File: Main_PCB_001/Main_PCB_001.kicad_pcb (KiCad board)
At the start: 4 copper layers, 55 x 15 mm, 65 parts, among them IC1 FDN8601, IC2 FDN8601, IC3 TPS40211QDGQRQ1, IC4 PAM2863ECR, IC5 FDN8601, IC6 ZXTR2105FQ-7, U1 ATtiny25-20S, U2 Mounting_Hole_M2, U3 Mounting_Hole_M2, U4 Mounting_Hole_M2, U5 Mounting_Hole_M2

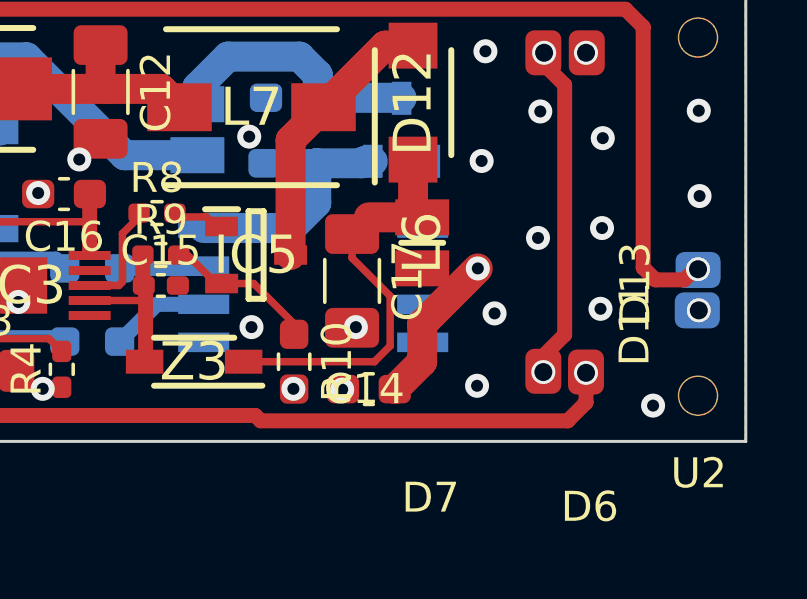
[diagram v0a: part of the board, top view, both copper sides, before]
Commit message: Corrections 001
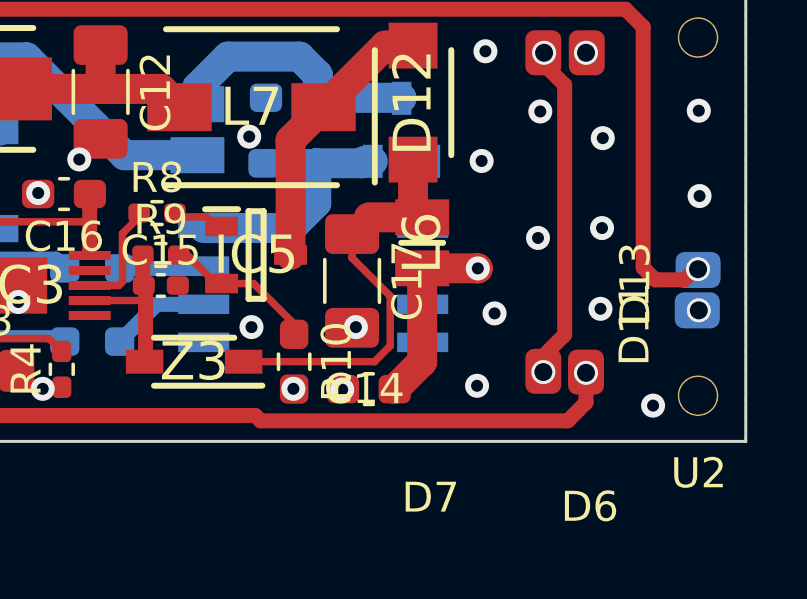
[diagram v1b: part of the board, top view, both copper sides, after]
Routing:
- net Net-(C14-Pad1): track 15.5 -> 16.6 mm
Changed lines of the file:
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@@
   (segment (start 133.7564 102.2958) (end 135.522 102.2958) (width 1) (layer "F.Cu") (net 10))
   (segment (start 135.522 102.2958) (end 136.1316 102.9054) (width 1) (layer "F.Cu") (net 10))
-  (segment (start 146.0754 108.2802) (end 144.2212 110.1344) (width 1) (layer "F.Cu") (net 11))
-  (segment (start 144.2212 110.1344) (end 144.2212 111.3879) (width 1) (layer "F.Cu") (net 11))
+  (segment (start 144.2212 108.2766) (end 144.2212 111.3879) (width 1) (layer "F.Cu") (net 11))
   (segment (start 144.2212 111.3879) (end 143.3057 112.3034) (width 1) (layer "F.Cu") (net 11))
+  (segment (start 146.0754 108.2802) (end 146.0718 108.2766) (width 1) (layer "F.Cu") (net 11))
+  (segment (start 146.0718 108.2766) (end 144.2212 108.2766) (width 1) (layer "F.Cu") (net 11))
   (via (at 146.0754 108.2802) (size 0.8) (drill 0.4) (layers "F.Cu" "B.Cu") (net 11))
   (via (at 149.6822 101.092) (size 0.8) (drill 0.6) (layers "F.Cu" "B.Cu") (net 11))

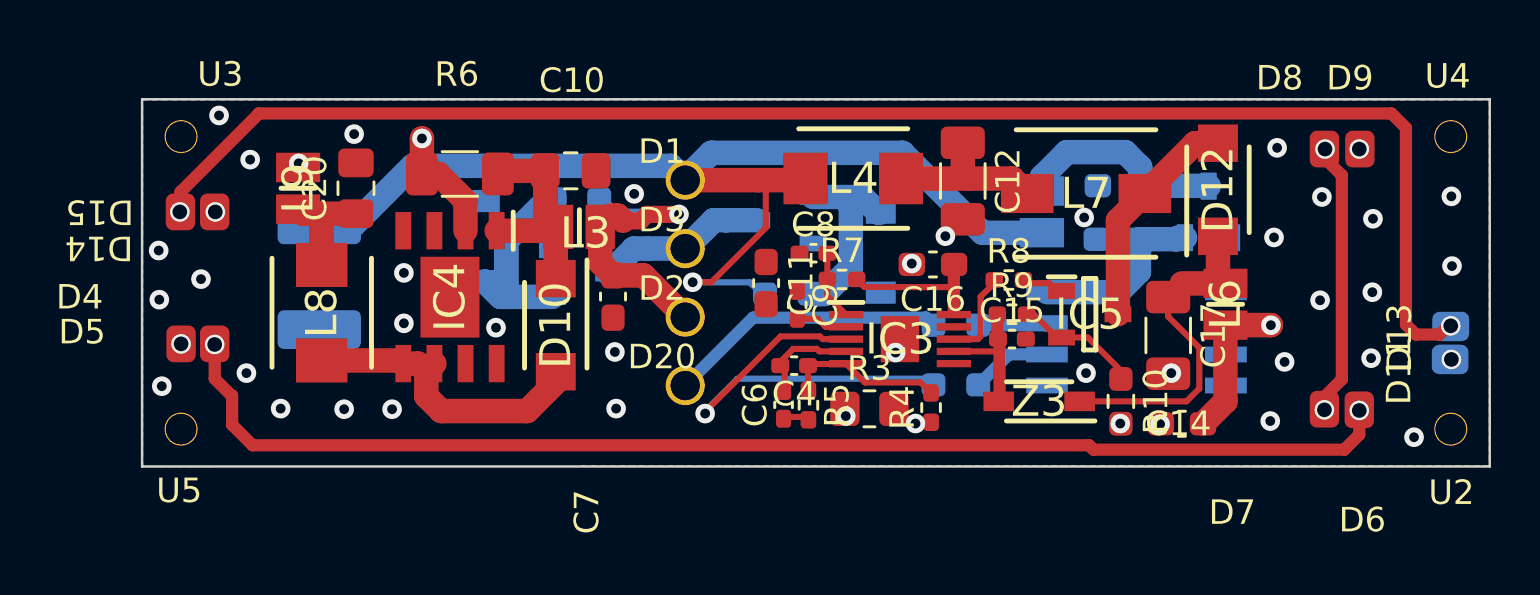
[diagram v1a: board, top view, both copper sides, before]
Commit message: Corrections 001
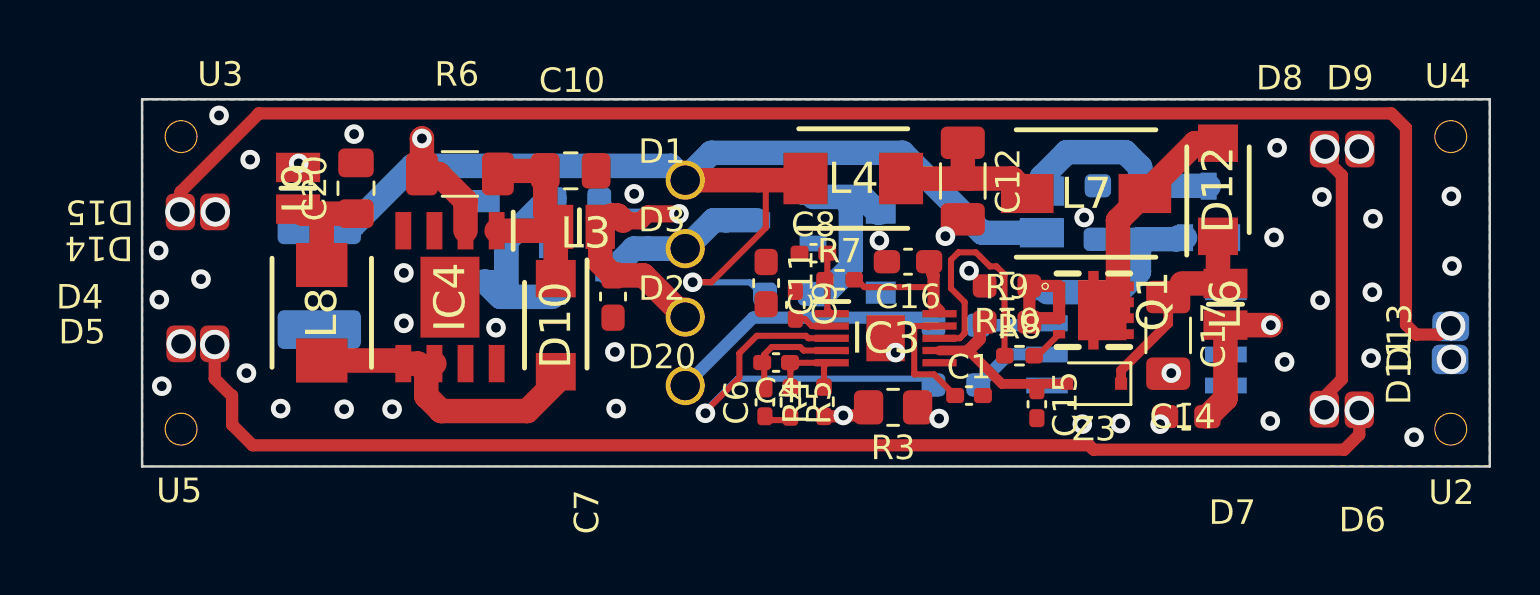
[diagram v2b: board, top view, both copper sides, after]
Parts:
- removed IC5: FDN8601, libraries:SOT95P251X112-3N
- added C1: C, Capacitor_SMD:C_0402_1005Metric_Pad0.74x0.62mm_HandSolder, F.Cu at (133.8, 111.2)
- added Q1: AON7407, libraries:DFN_3X3_EP, F.Cu at (138.8, 107.7)
- R9: footprint Resistor_SMD:R_0402_1005Metric_Pad0.72x0.64mm_HandSolder -> Resistor_SMD:R_0603_1608Metric_Pad0.98x0.95mm_HandSolder
- Z3: footprint libraries:SOD3616X130N -> Diode_SMD:D_SOD-323F
- moved R10 6.62 mm to (135.3, 106.7), turned to 180 degrees
- moved R4 4.38 mm to (127.8, 111.4)
- moved R8 3.12 mm to (135.8, 109.5)
- moved C15 2.84 mm to (136.5, 111.5), turned to -90 degrees
- moved Z3 2.36 mm to (138.9, 110.7)
- moved C16 1.02 mm to (131.3, 105.7)
- moved R3 0.97 mm to (130.7, 111.6), turned to 180 degrees
- moved C6 0.77 mm to (125.4, 111.4)
- moved C4 0.75 mm to (125.9, 109.8)
- moved R5 0.75 mm to (126.5, 111.4)
- moved IC3 0.59 mm to (130.4, 108.8)
- moved R9 0.38 mm to (135.3, 108.2)
- moved C14 0.34 mm to (142.6, 112.0)
- moved R7 0.10 mm to (128.5, 106.4)
- moved C9 0.08 mm to (126.7, 107.5)
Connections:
- IC3 pad 9: unconnected-(IC3-Pad9) -> Net-(IC3-Pad9)
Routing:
- net Net-(IC3-Pad8): track 3.54 -> 10.3 mm
- net Net-(IC3-Pad9): track 0.00 -> 5.14 mm
- net Net-(C17-Pad1): track 13.9 -> 8.86 mm
- net Net-(C4-Pad1): track 6.60 -> 4.02 mm
- net Net-(D4-Pad1): track 34.8 -> 32.2 mm
- net Net-(C15-Pad1): track 5.50 -> 7.39 mm
- net Net-(C16-Pad1): track 6.15 -> 5.33 mm
- net Net-(C9-Pad2): track 2.13 -> 1.60 mm
- net GND: vias 38 -> 39
